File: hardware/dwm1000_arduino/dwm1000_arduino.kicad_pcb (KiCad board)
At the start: 2 copper layers, 66 x 76.2 mm, 29 parts, among them J1 RAW_PWR, J2 PWR_IN, J3 UART, J4 SPI, J5 NEO_OUT, J6 DEBUG

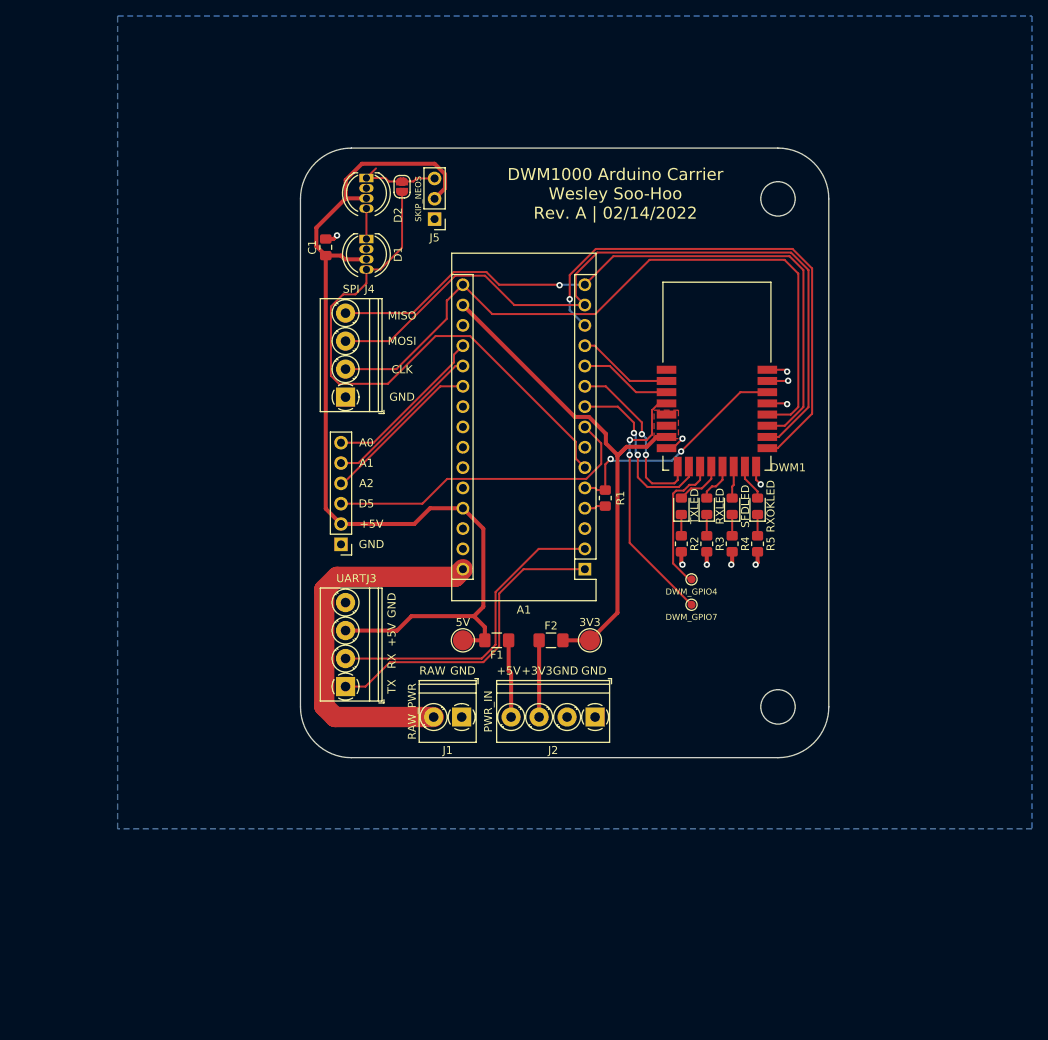
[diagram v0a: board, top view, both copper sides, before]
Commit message: finish layout
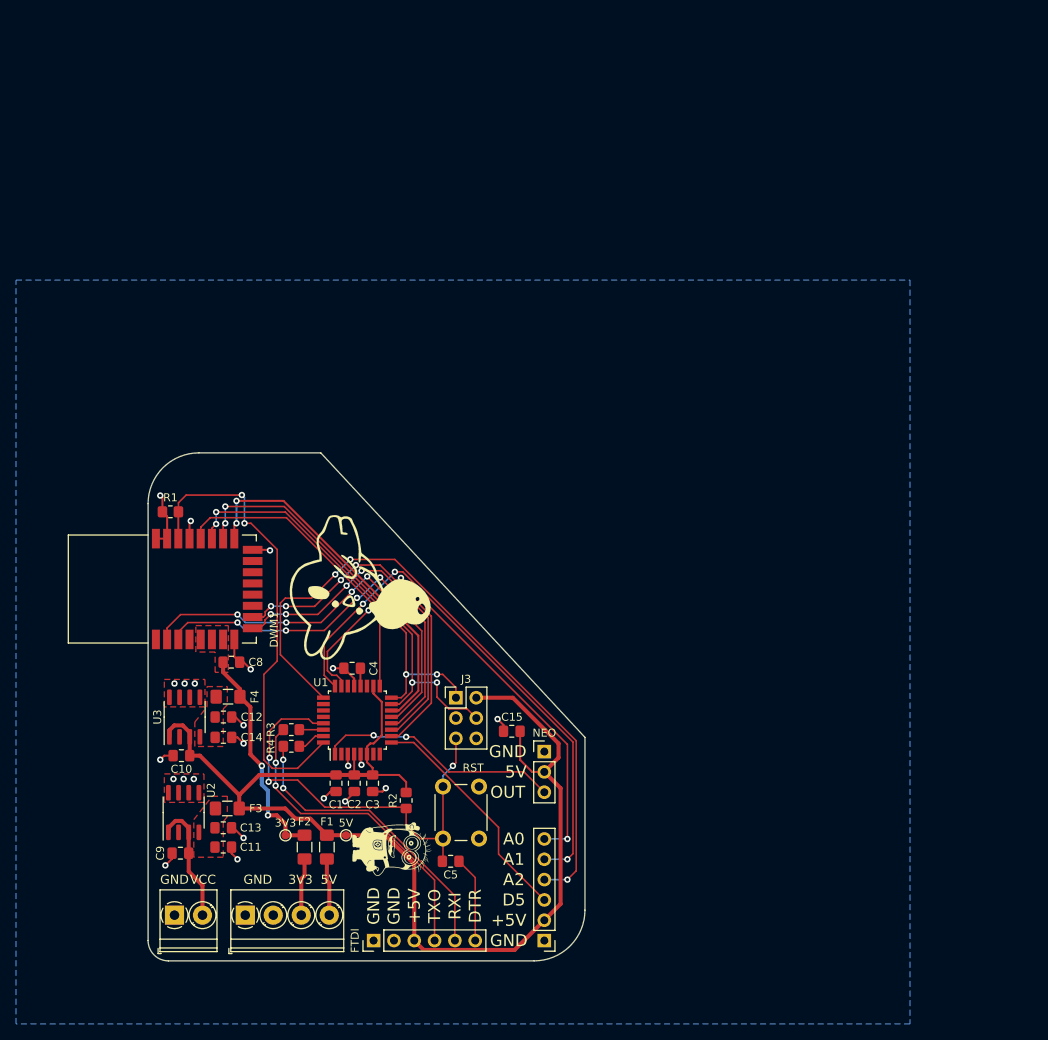
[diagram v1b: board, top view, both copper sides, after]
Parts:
- removed A1: Arduino_Nano, Module:Arduino_Nano
- removed D1, D2: NeoPixel_THT, LED_THT:LED_D5.0mm-4_RGB
- removed D3: TXLED, LED_SMD:LED_0805_2012Metric_Pad1.15x1.40mm_HandSolder
- removed D4: RXLED, LED_SMD:LED_0805_2012Metric_Pad1.15x1.40mm_HandSolder
- removed D5: SFDLED, LED_SMD:LED_0805_2012Metric_Pad1.15x1.40mm_HandSolder
- removed D6: RXOKLED, LED_SMD:LED_0805_2012Metric_Pad1.15x1.40mm_HandSolder
- removed J4: SPI, TerminalBlock_Phoenix:TerminalBlock_Phoenix_PT-1,5-4-3.5-H_1x04_P3.50mm_Horizontal
- removed J5: NEO_OUT, Connector_PinHeader_2.54mm:PinHeader_1x03_P2.54mm_Vertical
- removed JP1: SKIP_NEOS, Jumper:SolderJumper-2_P1.3mm_Open_RoundedPad1.0x1.5mm
- removed R5: 200, Resistor_SMD:R_0805_2012Metric_Pad1.20x1.40mm_HandSolder
- removed REF** (x2): MountingHole_4.3mm_M4, MountingHole:MountingHole_4.3mm_M4
- removed TP3: DWM_GPIO7, TestPoint:TestPoint_Pad_D1.0mm
- removed TP4: DWM_GPIO4, TestPoint:TestPoint_Pad_D1.0mm
- added C10: 1uF, Capacitor_SMD:C_0805_2012Metric_Pad1.18x1.45mm_HandSolder, F.Cu at (96.9, 130.6)
- added C11: 1uF, Capacitor_SMD:C_0805_2012Metric_Pad1.18x1.45mm_HandSolder, F.Cu at (102.1, 142.0)
- added C12: 1uF, Capacitor_SMD:C_0805_2012Metric_Pad1.18x1.45mm_HandSolder, F.Cu at (102.1, 125.7)
- added C13: 4.7uF, Capacitor_SMD:C_0805_2012Metric_Pad1.18x1.45mm_HandSolder, F.Cu at (102.1, 139.6)
- added C14: 4.7uF, Capacitor_SMD:C_0805_2012Metric_Pad1.18x1.45mm_HandSolder, F.Cu at (102.1, 128.3)
- added C15: 10uF, Capacitor_SMD:C_0805_2012Metric_Pad1.18x1.45mm_HandSolder, F.Cu at (138.2, 127.5)
- added C2: 1uF, Capacitor_SMD:C_0805_2012Metric_Pad1.18x1.45mm_HandSolder, F.Cu at (118.5, 134.0)
- added C3: 0.1uF, Capacitor_SMD:C_0805_2012Metric_Pad1.18x1.45mm_HandSolder, F.Cu at (120.8, 134.0)
- added C4: 0.1uF, Capacitor_SMD:C_0805_2012Metric_Pad1.18x1.45mm_HandSolder, F.Cu at (118.2, 119.6)
- added C5: 0.1uF, Capacitor_SMD:C_0805_2012Metric_Pad1.18x1.45mm_HandSolder, F.Cu at (130.5, 143.8)
- added C8: 1uF, Capacitor_SMD:C_0805_2012Metric_Pad1.18x1.45mm_HandSolder, F.Cu at (103.1, 118.9)
- added C9: 1uF, Capacitor_SMD:C_0805_2012Metric_Pad1.18x1.45mm_HandSolder, F.Cu at (96.8, 142.7)
- added F3: 500mA, Fuse:Fuse_1206_3216Metric_Pad1.42x1.75mm_HandSolder, F.Cu at (102.6, 137.2)
- added F4: 500mA, Fuse:Fuse_1206_3216Metric_Pad1.42x1.75mm_HandSolder, F.Cu at (102.7, 123.2)
- added FTDI: UART/FTDI, Connector_PinHeader_2.54mm:PinHeader_1x06_P2.54mm_Vertical, F.Cu at (120.9, 153.7)
- added G***: LOGO, wsh:mimi_heart, F.Cu at (119.4, 109.9)
- added G***: LOGO, wsh:minion, F.Cu at (123.2, 142.2)
- added G***: LOGO, wsh:mimi_melon, B.Cu at (118.7, 127.6)
- added G***: LOGO, wsh:surprised_pika, B.Cu at (143.5, 141.0)
- added NEO: NEO_OUT, Connector_PinHeader_2.54mm:PinHeader_1x03_P2.54mm_Vertical, F.Cu at (142.2, 130.0)
- added RST: RST, Button_Switch_THT:SW_PUSH_6mm, F.Cu at (134.1, 134.4)
- added U1: ATmega328P-A, Package_QFP:TQFP-32_7x7mm_P0.8mm, F.Cu at (118.9, 126.1)
- added U2: MIC5239-5.0YM-TR, Package_SO:SOIC-8_3.9x4.9mm_P1.27mm, F.Cu at (97.2, 137.7)
- added U3: MIC5239-3.3YM, Package_SO:SOIC-8_3.9x4.9mm_P1.27mm, F.Cu at (97.3, 125.7)
- C1: value 10uF -> 1uF
- J2: value PWR_IN -> PWR_OUT
- J3: value UART -> AVR ICSP; footprint TerminalBlock_Phoenix:TerminalBlock_Phoenix_PT-1,5-4-3.5-H_1x04_P3.50mm_Horizontal -> Connector_PinHeader_2.54mm:PinHeader_2x03_P2.54mm_Vertical
- R2: value 200 -> 10K
- R3, R4: value 200 -> 1K
- TP1, TP2: footprint TestPoint:TestPoint_Pad_D2.5mm -> TestPoint:TestPoint_Pad_D1.0mm
- moved DWM1 74.3 mm to (94.5, 109.7), turned to 90 degrees
- moved C1 67.0 mm to (116.2, 134.0), turned to -90 degrees
- moved R4 60.6 mm to (110.6, 129.4), turned to 180 degrees
- moved R3 56.9 mm to (110.6, 127.3), turned to 0 degrees
- moved J6 55.7 mm to (142.2, 153.7)
- moved R1 54.4 mm to (95.5, 100.1), turned to 180 degrees
- moved J2 50.3 mm to (104.9, 150.5), turned to 0 degrees
- moved R2 47.0 mm to (125.0, 136.2), turned to 90 degrees
- moved TP2 45.2 mm to (109.9, 140.5)
- moved J1 43.6 mm to (96.0, 150.5), turned to 0 degrees
- moved F2 40.2 mm to (112.3, 142.0), turned to 90 degrees
- moved F1 33.4 mm to (115.1, 142.0), turned to 90 degrees
- moved TP1 28.4 mm to (117.4, 140.5)
- moved J3 13.9 mm to (131.2, 123.3), turned to 0 degrees
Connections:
- DWM1 pad 11: Net-(DWM1-Pad11) -> unconnected-(DWM1-Pad11)
- DWM1 pad 12: DWM_TXLED -> unconnected-(DWM1-Pad12)
- DWM1 pad 13: DWM_RXLED -> unconnected-(DWM1-Pad13)
- DWM1 pad 14: DWM_SFDLED -> unconnected-(DWM1-Pad14)
- DWM1 pad 15: DWM_RXOKLED -> unconnected-(DWM1-Pad15)
- DWM1 pad 4: Net-(DWM1-Pad4) -> unconnected-(DWM1-Pad4)
- J3 pad 1: ARD_TX -> SPI_MISO
- J3 pad 2: ARD_RX -> +5V
- J3 pad 3: +5V -> SPI_SCK
- J3 pad 4: GND -> SPI_MOSI
- J6 pad 3: ARD_D5 -> AVR_D5
- J6 pad 4: ARD_A2 -> AVR_A2
- J6 pad 5: ARD_A1 -> AVR_A1
- J6 pad 6: ARD_A0 -> AVR_A0
- R2 pad 1: Net-(D3-Pad1) -> ~{AVR_RST}
- R2 pad 2: GND -> +5V
- R3 pad 1: Net-(D4-Pad1) -> AVR_RX
- R3 pad 2: GND -> Net-(R3-Pad2)
- R4 pad 2: GND -> AVR_TX
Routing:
- net AVR_A2: track 0.00 -> 83.4 mm, vias 0 -> 3
- net AVR_A1: track 0.00 -> 67.4 mm, vias 0 -> 3
- net AVR_A0: track 0.00 -> 62.5 mm, vias 0 -> 3
- net ~{AVR_RST}: track 0.00 -> 56.2 mm, vias 0 -> 3
- net SPI_CLK: track 88.3 -> 38.5 mm
- net /MCUs/~{DWM_RST}: track 11.6 -> 52.6 mm, vias 0 -> 4
- net NEO_DATA: track 71.2 -> 30.7 mm, vias 0 -> 2
- net /MCUs/DWM_WAKE: track 12.0 -> 52.3 mm, vias 0 -> 4
- net ARD_D5: track 40.1 -> 0.00 mm
- net AVR_RX: track 0.00 -> 39.9 mm, vias 0 -> 2
- net ARD_TX: track 39.9 -> 0.00 mm
- net ARD_RX: track 39.5 -> 0.00 mm
- net SPI_MOSI: track 94.1 -> 55.4 mm, vias 0 -> 4
- net AVR_TX: track 0.00 -> 37.9 mm, vias 0 -> 2
- net +3V3: track 64.2 -> 27.9 mm, vias 0 -> 2
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- added copper zone on F.Cu, net /Power/3V3_UNFUSED
- added copper zone on F.Cu, net /Power/5V_UNFUSED
- added copper zone on F.Cu, net GND
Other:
- board size 66 x 76.2 mm -> 54.6 x 63.5 mm
- board text added: "3V3"
- board text added: "5V"
- board text added: "DTR"
- board text added: "DWM1000 AVR Dev Board Wesley Soo-Hoo Rev. B | 2022/04/10"
- board text added: "OUT"
- board text added: "RXI"
- board text added: "TXO"
- board text added: "VCC"
- board text removed: "+3V3"
- board text removed: "CLK"
- board text removed: "DWM1000 Arduino Carrier Wesley Soo-Hoo Rev. A | 02/14/2022"
- board text removed: "MISO"
- board text removed: "MOSI"
- board text removed: "RAW"
- board text removed: "RX"
- board text removed: "TX"
